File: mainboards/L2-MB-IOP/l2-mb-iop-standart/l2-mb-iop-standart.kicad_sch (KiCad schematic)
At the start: 46 parts, among them J1 URP_Conn_01x12_Socket, J10 GPP_Conn_01x12_Socket, J11 GPP_Conn_01x12_Socket, J12 GPP_Conn_01x12_Socket, J13 GPP_Conn_01x12_Socket, J14 GPP_Conn_01x12_Socket, J15 AIP_Conn_01x12_Socket, J16 AIP_Conn_01x12_Socket, J17 AIP_Conn_01x12_Socket, J18 AIP_Conn_01x12_Socket, J19 ICP_Conn_01x12_Socket, J2 URP_Conn_01x12_Socket, J20 ICP_Conn_01x12_Socket, J21 AIP_Conn_01x12_Socket, J22 AIP_Conn_01x12_Socket, J23 Conn_01x03_Pin, J24 Conn_01x02_Pin, J25 Conn_01x02_Pin, J26 Conn_01x02_Pin, J27 Conn_01x02_Pin, J28 Conn_01x02_Pin, J29 Conn_01x02_Pin, J3 GPP_Conn_01x12_Socket, J4 GPP_Conn_01x12_Socket, J5 GPP_Conn_01x12_Socket, J6 GPP_Conn_01x12_Socket, J7 GPP_Conn_01x12_Socket, J8 GPP_Conn_01x12_Socket, J9 GPP_Conn_01x12_Socket, SW1 SW_SPDT, U1 LM2596s_module, U2 LM2596_mini_module

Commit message: Board first version
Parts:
- removed C1, C3: C, Capacitor_THT:C_Disc_D4.3mm_W1.9mm_P5.00mm, symbol Device:C
- removed C5, C7: C_Polarized, Capacitor_THT:CP_Radial_D6.3mm_P2.50mm, symbol Device:C_Polarized
- removed D2: D_Schottky, Diode_THT:D_DO-15_P10.16mm_Horizontal, symbol Device:D_Schottky
- removed J24, J25, J26, J27, J28, J29: Conn_01x02_Pin, Connector_PinHeader_2.54mm:PinHeader_1x02_P2.54mm_Vertical, symbol Connector:Conn_01x02_Pin
- removed PS2: B240XS-2W, tuxmio:B240XS-2W, symbol tuxmio:B240XS-2W
- removed SW1: SW_SPDT, tuxmio:SW-SPDT_1x03_P2.54mm_Vertical, symbol Switch:SW_SPDT
- removed U1: LM2596s_module, tuxmio:LM2596s_module, symbol tuxmio:LM2596s_module
- removed U2: LM2596_mini_module, tuxmio:LM2596_mini_module, symbol tuxmio:LM2596_mini_module
- added J10, J11, J12, J13, J2, J3, J4, J5, J6, J7, J8, J9: Conn_01x01_Pin, Connector_PinHeader_1.00mm:PinHeader_1x01_P1.00mm_Vertical, symbol Connector:Conn_01x01_Pin
- J1: renamed from J23; footprint Connector_Phoenix_MC_HighVoltage:PhoenixContact_MCV_1,5_3-G-5.08_1x03_P5.08mm_Vertical -> Connector_PinHeader_2.54mm:PinHeader_1x03_P2.54mm_Vertical
- renumbered C2 to C1, C6 to C2, C4 to C3, C8 to C4, J1 to J14, J2 to J15, J3 to J16, J4 to J17, J5 to J18, J6 to J19, J7 to J20, J8 to J21, J9 to J22, J10 to J23, J11 to J24, J12 to J25, J13 to J26, J14 to J27, J15 to J28, J16 to J29, J17 to J30, J18 to J31, J19 to J32, J20 to J33, J21 to J34, J22 to J35, PS3 to PS2
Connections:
- net +5V: now also J10.1 (Pin_1), J12.1 (Pin_1), J6.1 (Pin_1)
- net 0V_bipolar: now also J5.1 (Pin_1)
- net GND: now also J3.1 (Pin_1), J4.1 (Pin_1)
- net GND1: now also J2.1 (Pin_1), J9.1 (Pin_1)
- net at A1.18 (AREF), J28.2 (A_Ref), J29.2 (A_Ref)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: now also J7.1 (Pin_1)
- net at J1.1 (Pin_1): now also D1.2 (A)
- net at A1.28 (~{RESET}): now also J8.1 (Pin_1)
- net at A1.30 (VIN): now also J13.1 (Pin_1)
- net at A1.17 (3V3): now also J11.1 (Pin_1)
- no-connect marks 61 -> 60
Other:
- note added: "note for future Mega 2560 has 54 digital input/output pins, of which 14 can be used for PWM output. + It also has 16 analog input pins in addition. End part 2x18-2x5V-2xGND"
- note removed: "note for future Mega 2560 has 54 digital input/output pins, of which 14 can be used for PWM output. + It also has 16 analog input pins in addition."
- moved on the sheet: C3, C4, PS2

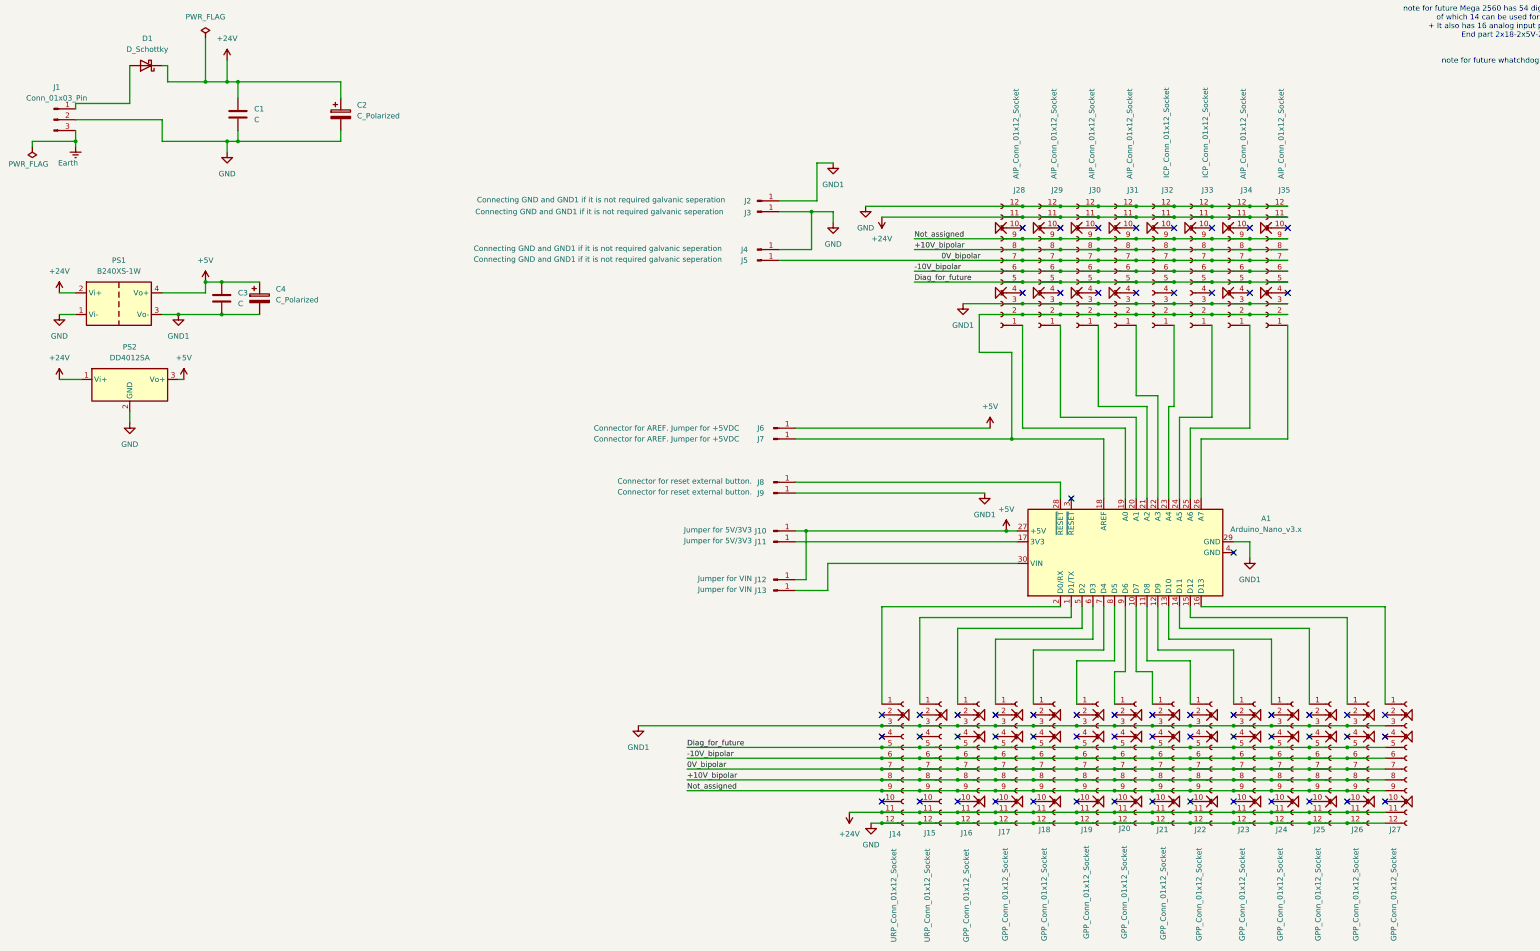
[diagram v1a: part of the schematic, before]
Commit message: Started first DO board
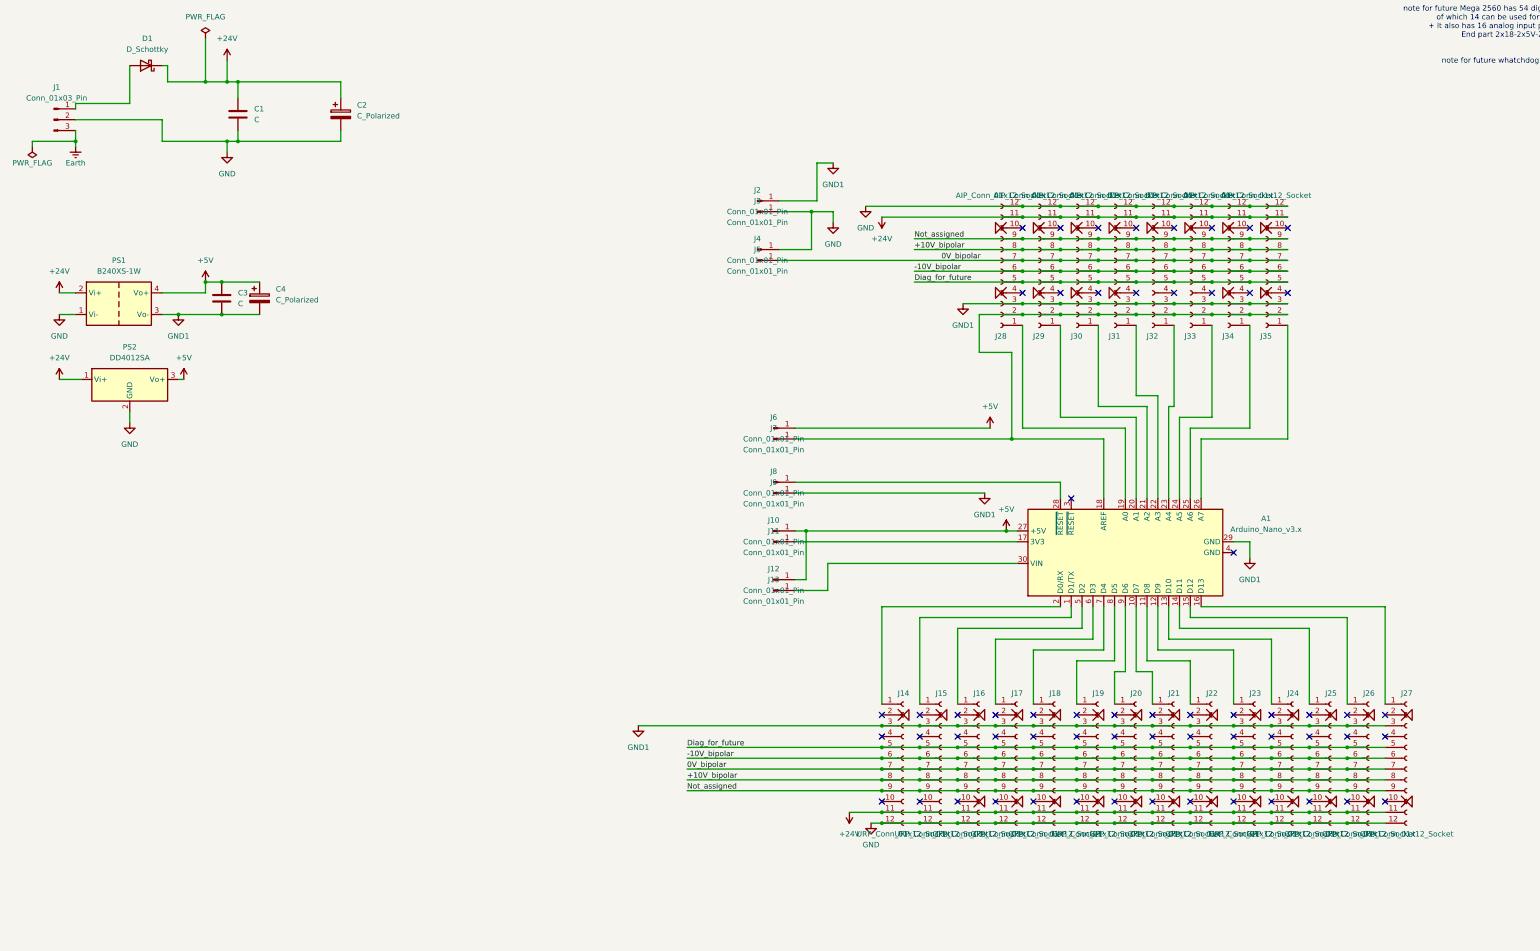
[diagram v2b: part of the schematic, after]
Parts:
- C1, C3: footprint Capacitor_SMD:C_0805_2012Metric_Pad1.18x1.45mm_HandSolder -> (none)
- C2, C4: footprint Capacitor_SMD:CP_Elec_4x5.3 -> (none)
- D1: footprint Diode_SMD:D_1206_3216Metric -> (none)
- J1: footprint Connector_PinHeader_2.54mm:PinHeader_1x03_P2.54mm_Vertical -> (none)
- J10, J11, J12, J13, J2, J3, J4, J5, J6, J7, J8, J9: footprint Connector_PinHeader_1.00mm:PinHeader_1x01_P1.00mm_Vertical -> (none)
- J14, J15: footprint tuxmio:MB_URP_socket_PinHeader_1x12_P2.54mm_Vertical -> tuxmio:MB_URP_PinSocket_1x12_P2.54mm_Vertical
- J16, J17, J18, J19, J20, J21, J22, J23, J24, J25, J26, J27: footprint tuxmio:MB_GPP_socket_PinHeader_1x12_P2.54mm_Vertical -> tuxmio:MB_GPP_PinSocket_1x12_P2.54mm_Vertical
- J28, J29, J30, J31, J34, J35: footprint tuxmio:MB_AIP_socket_PinHeader_1x12_P2.54mm_Vertical -> tuxmio:MB_AIP_PinSocket_1x12_P2.54mm_Vertical
- J32, J33: footprint tuxmio:MB_ICP_socket_PinHeader_1x12_P2.54mm_Vertical -> tuxmio:MB_ICP_PinSocket_1x12_P2.54mm_Vertical
